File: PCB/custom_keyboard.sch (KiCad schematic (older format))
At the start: 403 parts, among them IC1 FE2.1, J1 USB_A, J2 USB_A, J3 USB_A, J4 Conn_01x08_Male, SW1 SW_Push, U1 PRTR5V0U2X, U2 24LC02, U3 PRTR5V0U2X, U4 PRTR5V0U2X, U5 PRTR5V0U2X, U6 PRTR5V0U2X, U7 PRTR5V0U2X, U8 PRTR5V0U2X, U9 AT90USB646-MU, Y1 12MHz, Y2 16MHz

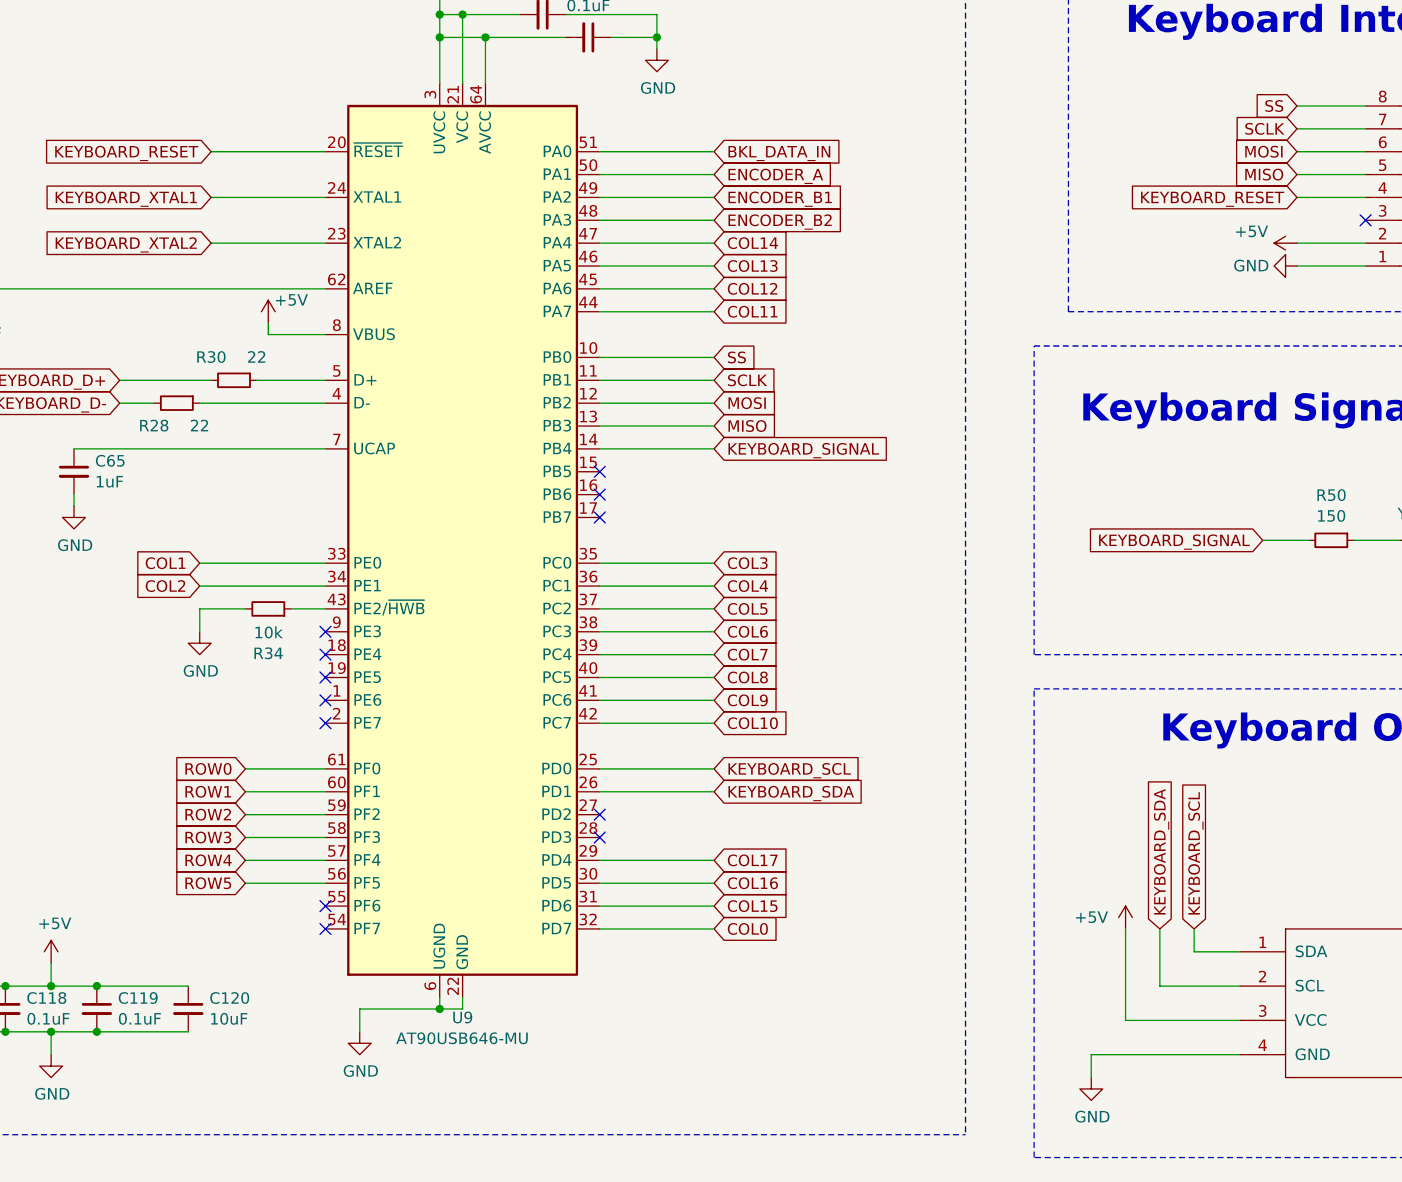
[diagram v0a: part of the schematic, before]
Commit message: LED routing
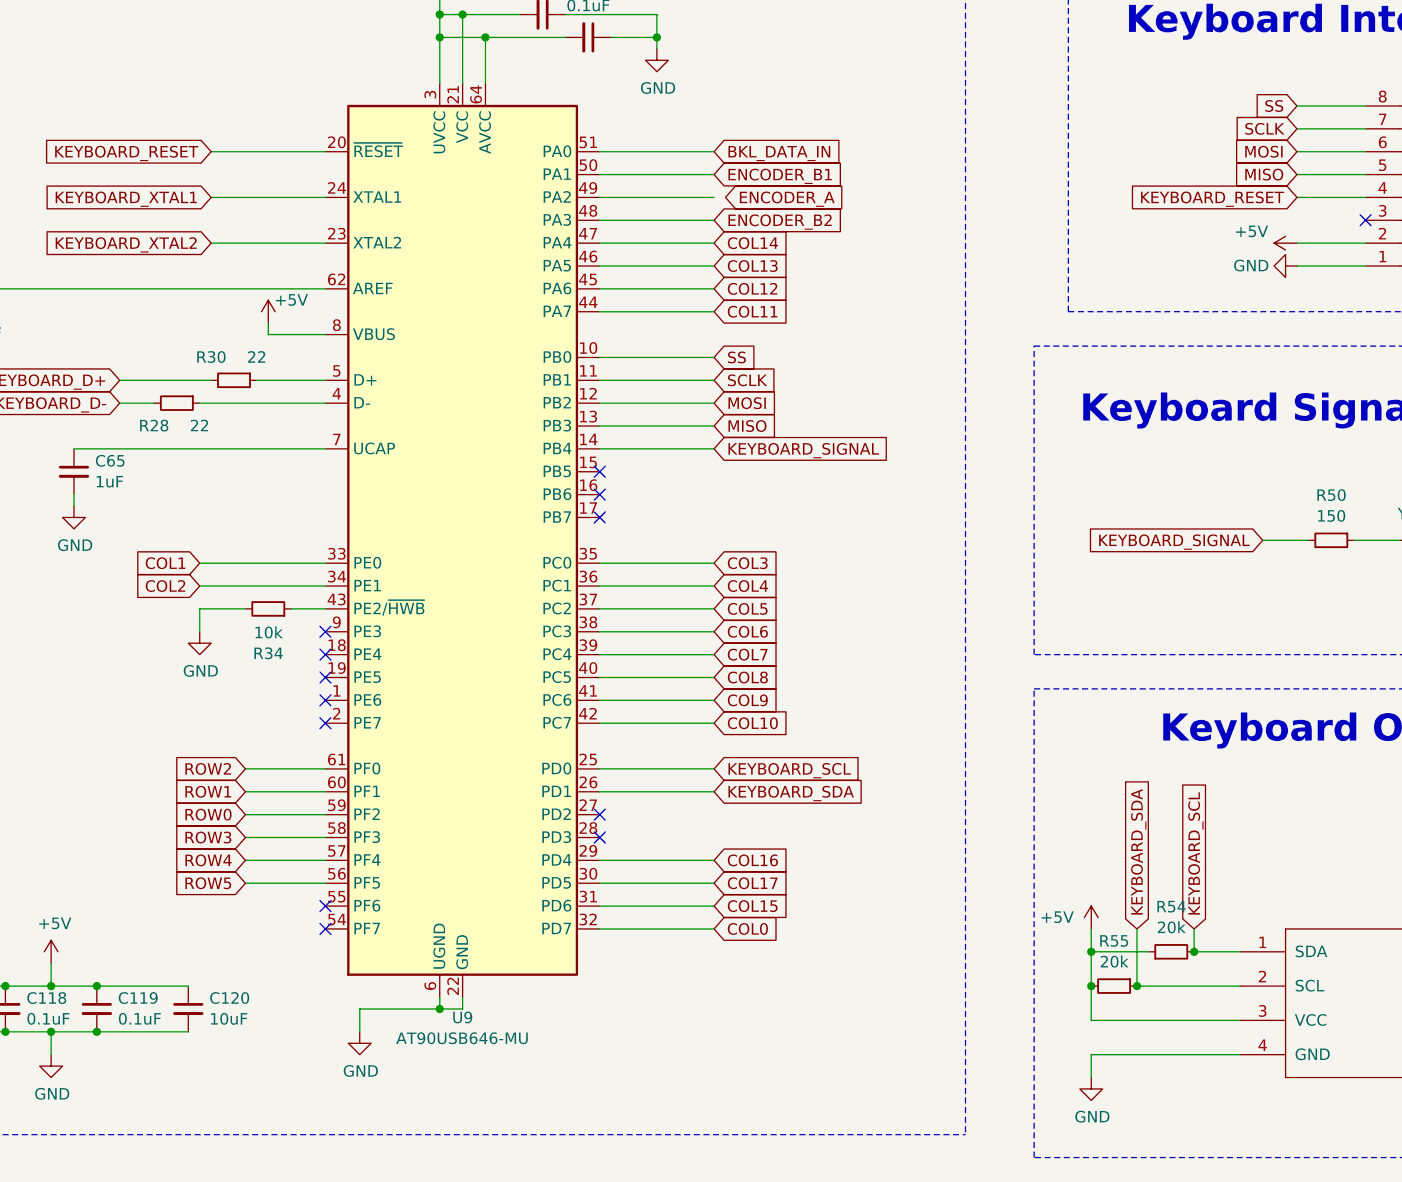
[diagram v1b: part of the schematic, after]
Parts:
- added R54, R55: 20k, Resistor_SMD:R_0805_2012Metric, symbol Device:R_Small
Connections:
- net +5V: now also R54.1, R55.2
- net COL16: now also U9.29 (PD4); no longer U9.30 (PD5)
- net COL17: now also U9.30 (PD5); no longer U9.29 (PD4)
- net ENCODER_A: no longer U9.50 (PA1)
- net ENCODER_B1: now also U9.50 (PA1); no longer U9.49 (PA2)
- net KEYBOARD_SCL: now also R54.2
- net KEYBOARD_SDA: now also R55.1
- net ROT1_ROW: now also U9.59 (PF2); no longer U9.61 (PF0)
- net ROW2: now also U9.61 (PF0); no longer U9.59 (PF2)
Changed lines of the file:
@@
 	1    0    0    -1
 $EndComp
-Text GLabel 9650 19250 1    50   Input ~ 0
+Text GLabel 9550 19250 1    50   Input ~ 0
 KEYBOARD_SDA
 Text GLabel 9800 19250 1    50   Input ~ 0
@@
 L power:+5V #PWR0197
 U 1 1 745E23C2
-P 9500 19250
-F 0 "#PWR0197" H 9500 19100 50  0001 C CNN
-F 1 "+5V" H 9350 19300 50  0000 C CNN
-F 2 "" H 9500 19250 50  0001 C CNN
-F 3 "" H 9500 19250 50  0001 C CNN
-	1    9500 19250
+P 9350 19250
+F 0 "#PWR0197" H 9350 19100 50  0001 C CNN
+F 1 "+5V" H 9200 19300 50  0000 C CNN
+F 2 "" H 9350 19250 50  0001 C CNN
+F 3 "" H 9350 19250 50  0001 C CNN
+	1    9350 19250
 	1    0    0    -1
 $EndComp
@@
 	10000 19350 9800 19350
 Wire Wire Line
-	10000 19500 9650 19500
-Wire Wire Line
-	9500 19650 10000 19650
-Wire Wire Line
 	9350 19800 10000 19800
 Text Notes 9650 18450 0    118  ~ 24
@@
 	9800 19250 9800 19350
 Wire Wire Line
-	9500 19250 9500 19650
+	9350 19250 9350 19350
 Wire Wire Line
-	9650 19500 9650 19250
+	9550 19500 9550 19250
 Wire Wire Line
 	9350 19900 9350 19800
@@
 Wire Wire Line
 	7200 15850 7700 15850
-Text GLabel 7700 18950 2    50   Input ~ 0
-COL17
 Text GLabel 7700 19050 2    50   Input ~ 0
+COL17
+Text GLabel 7700 18950 2    50   Input ~ 0
 COL16
 Text GLabel 7700 19150 2    50   Input ~ 0
@@
 	1    0    0    -1
 $EndComp
-Text GLabel 5650 18550 0    50   Input ~ 0
+Text GLabel 5650 18750 0    50   Input ~ 0
 ROW0
 Text GLabel 5650 18650 0    50   Input ~ 0
 ROW1
-Text GLabel 5650 18750 0    50   Input ~ 0
+Text GLabel 5650 18550 0    50   Input ~ 0
 ROW2
 Text GLabel 5650 18850 0    50   Input ~ 0
@@
 BKL_DATA_IN
 Text GLabel 7700 15950 2    50   Input ~ 0
-ENCODER_A
-Text GLabel 7700 16050 2    50   Input ~ 0
 ENCODER_B1
 Text GLabel 7700 16150 2    50   Input ~ 0
@@
 Text GLabel 7700 17750 2    50   Input ~ 0
 COL4
+Text GLabel 7750 16050 2    50   Input ~ 0
+ENCODER_A
+$Comp
+L Device:R_Small R55
+U 1 1 A0A4D4B3
+P 9450 19500
+F 0 "R55" V 9254 19500 50  0000 C CNN
+F 1 "20k" V 9345 19500 50  0000 C CNN
+F 2 "Resistor_SMD:R_0805_2012Metric" H 9450 19500 50  0001 C CNN
+F 3 "~" H 9450 19500 50  0001 C CNN
+	1    9450 19500
+	0    1    1    0
+$EndComp
+Connection ~ 9550 19500
+Connection ~ 9350 19500
+Wire Wire Line
+	9350 19500 9350 19650
+$Comp
+L Device:R_Small R54
+U 1 1 A0A4DDB4
+P 9700 19350
+F 0 "R54" V 9896 19350 50  0000 C CNN
+F 1 "20k" V 9805 19350 50  0000 C CNN
+F 2 "Resistor_SMD:R_0805_2012Metric" H 9700 19350 50  0001 C CNN
+F 3 "~" H 9700 19350 50  0001 C CNN
+	1    9700 19350
+	0    -1   -1   0
+$EndComp
+Connection ~ 9800 19350
+Wire Wire Line
+	9550 19500 10000 19500
+Wire Wire Line
+	9350 19650 10000 19650
+Wire Wire Line
+	9600 19350 9350 19350
+Connection ~ 9350 19350
+Wire Wire Line
+	9350 19350 9350 19500
 $EndSCHEMATC
